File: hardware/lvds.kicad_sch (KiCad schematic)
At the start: 52 parts, among them U4 GateMate-CCGM1A1, Y1 ASE2-25.000MHZ-L-C-T

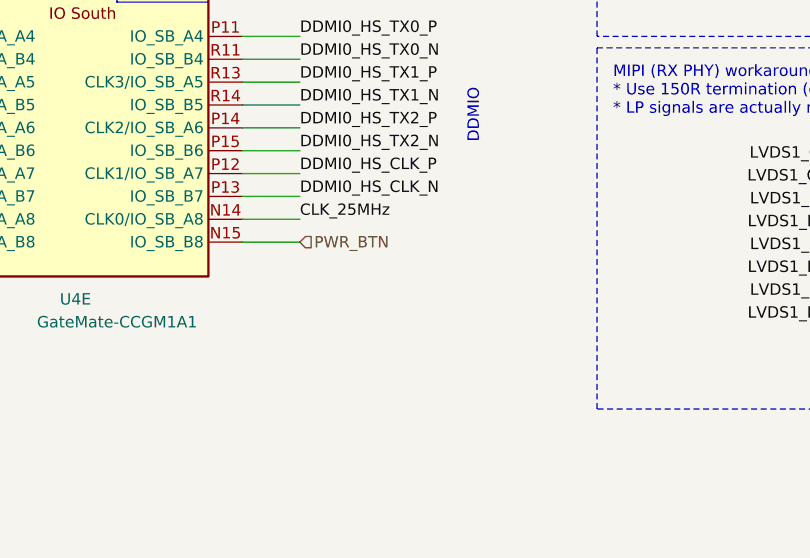
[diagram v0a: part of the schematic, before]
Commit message: Adding some tekst
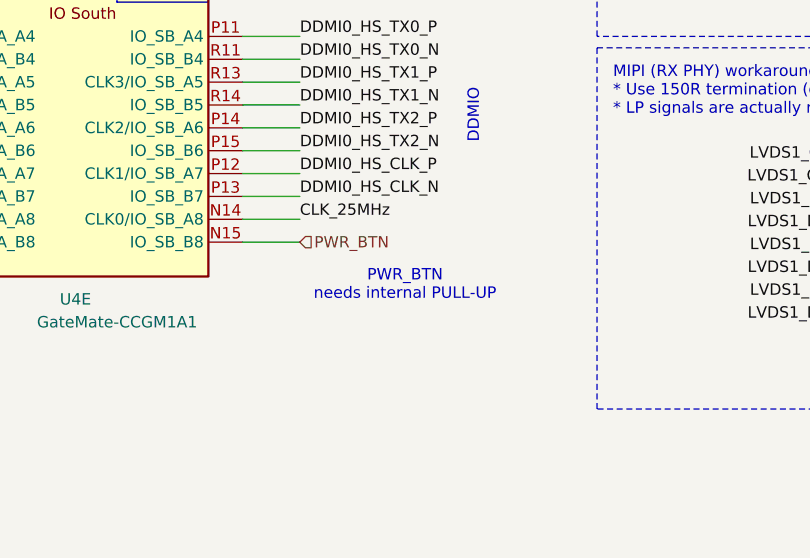
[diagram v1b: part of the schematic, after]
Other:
- note added: "PWR_BTN needs internal PULL-UP"
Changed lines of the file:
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@@
+		)
+	)
+	(text "PWR_BTN\nneeds internal PULL-UP"
+		(exclude_from_sim no)
+		(at 188.214 106.426 0)
+		(effects
+			(font
+				(size 1.27 1.27)
+			)
 		)
 	)
